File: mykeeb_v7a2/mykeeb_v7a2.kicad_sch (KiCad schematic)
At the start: 52 parts, among them SW43 SW_Push, SW44 SW_SPDT, U2 xiao-ble

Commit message: update
Signed-off-by: Maximilian Huber <gh@maxhbr.de>
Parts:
- added BT1: Battery_Cell, Connector_JST:JST_PH_S2B-PH-K_1x02_P2.00mm_Horizontal, symbol Device:Battery_Cell
- added D1, D11, D12, D13, D14, D15 (x2), D2, D3, D4 (x2), D6, D7, D8, D9: BAV70, Package_TO_SOT_SMD:SOT-23, symbol hillside_basic:BAV70_Small
- added S0, S1, S10, S11, S12, S13, S14, S15, S2, S20, S21, S22, S23, S24, S25, S3, S30 (x2), S31, S32, S33, S34, S35, S4, S43, S44, S45 (x2), S46: SW, pretty:MX-1U-Hotswap, symbol YAEMK:MX_1U
- added SW43: SW_Push, Button_Switch_SMD:SW_SPST_TL3342, symbol Switch:SW_Push
- added SW43: SW_Push, pretty:PushSW, symbol Switch:SW_Push
- added SW44: SW_SPDT, sepp:switch-MSK-12C02-smd, symbol Switch:SW_SPDT
- added U2: xiao-ble, pretty:xiao-ble-smd-cutout, symbol sepp:xiao-ble-geist
- SW43: footprint pretty:PushSW -> Button_Switch_SMD:SW_SPST_TL3342
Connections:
- net COL0: now also S0.2, S10.2, S20.2, S30.2, S30.2; no longer S0.1, S10.1, S20.1, S30.1, S30.1
- net COL1: now also S11.2, S21.1, S31.1, S43.1, SW43.1; no longer S11.1, S21.2, S31.2, S43.2, SW43.2
- net COL2: now also S12.1, S2.1, S22.2, S32.2, S44.2; no longer S12.2, S2.2, S22.1, S32.1, S44.1
- net COL3: now also S13.2, S23.1, S3.2, S33.1, S45.1; no longer S13.1, S23.2, S3.1, S33.2, S45.2
- net COL4: now also S14.1, S24.2, S34.2, S4.2, S46.2; no longer S14.2, S24.1, S34.1, S4.1, S46.1
- net COL5: now also S1.1, S15.2, S25.1, S35.1, S45.1; no longer S1.2, S15.1, S25.2, S35.2, S45.2
- net GND: now also BT1.2 (-), SW43.2, U2.13 (GND), U2.18 (GND), U2.20 (GND)
- net at D12.2 (A2): now also S15.1; no longer S15.2
- net at D4.1 (A1): now also S30.1; no longer S30.2 (x2)
- net at D4.2 (A2): now also S43.2; no longer S43.1
- net at D6.1 (A1): now also S2.2; no longer S2.1
- net at D6.2 (A2): now also S3.1; no longer S3.2
- net at D9.2 (A2): now also S33.2; no longer S33.1
- net at D2.2 (A2): now also S11.1; no longer S11.2
- net at D15.1 (A1): now also S44.1; no longer S44.2
- net at D12.1 (A1): now also S14.2; no longer S14.1
- net at D15.2 (A2): now also S45.2; no longer S45.1 (x2)
- net at D13.1 (A1): now also S24.1; no longer S24.2
- net at D13.2 (A2): now also S25.2; no longer S25.1
- net at D9.1 (A1): now also S32.1; no longer S32.2
- net at D2.1 (A1): now also S10.1; no longer S10.2
- net at D11.1 (A1): now also S4.1; no longer S4.2
- net at D11.2 (A2): now also S1.2; no longer S1.1
- net at D1.2 (A2): now also SW43.2; no longer SW43.1
- net at D8.1 (A1): now also S22.1; no longer S22.2
- net at D8.2 (A2): now also S23.2; no longer S23.1
- net at D14.1 (A1): now also S34.1; no longer S34.2
- net at D14.2 (A2): now also S35.2; no longer S35.1
- net at D3.1 (A1): now also S20.1; no longer S20.2
- net at D1.1 (A1): now also S0.1; no longer S0.2
- net at D15.1 (A1): now also S46.1; no longer S46.2
- net at D7.1 (A1): now also S12.2; no longer S12.1
- net at D4.2 (A2): now also S31.2; no longer S31.1
- net at D3.2 (A2): now also S21.2; no longer S21.1
- net at D7.2 (A2): now also S13.1; no longer S13.2
- new net: D8.1 (A1), S22.2
- new net: D8.2 (A2), S23.1
- new net: D12.2 (A2), S15.2
- new net: D11.1 (A1), S4.2
- new net: D4.1 (A1), S30.2 (x2)
- new net: D4.2 (A2), S43.1
- new net: D3.2 (A2), S21.1
- new net: D7.1 (A1), S12.1
- new net: D6.1 (A1), S2.1
- new net: D6.2 (A2), S3.2
- new net: D11.2 (A2), S1.1
- new net: D13.1 (A1), S24.2
- new net: D13.2 (A2), S25.1
- new net: D12.1 (A1), S14.1
- new net: D1.1 (A1), S0.2
- new net: D1.2 (A2), SW43.1
- new net: D14.2 (A2), S35.1
- new net: D2.1 (A1), S10.2
- new net: D2.2 (A2), S11.2
- new net: D7.2 (A2), S13.2
- new net: D15.2 (A2), S45.1 (x2)
- new net: D9.1 (A1), S32.2
- new net: D4.2 (A2), S31.1
- new net: D15.1 (A1), S46.2
- new net: D9.2 (A2), S33.1
- new net: D14.1 (A1), S34.2
- new net: D15.1 (A1), S44.2
- new net: D3.1 (A1), S20.2
- new net L_BAT+: SW44.2 (B), U2.19 (BAT)
- new net L_COL0: S0.1, S10.1, S20.1, S30.1, S30.1, U2.11 (A6_MOSI/1.15)
- new net L_COL1: S11.1, S21.2, S31.2, S43.2, SW43.2, U2.10 (A5_MISO/1.14)
- new net L_COL2: S12.2, S2.2, S22.1, S32.1, S44.1, U2.9 (A7_SCK/1.13)
- new net L_COL3: S13.1, S23.2, S3.1, S33.2, S45.2, U2.8 (B9_RX/1.12)
- new net L_COL4: S14.2, S24.1, S34.1, S4.1, S46.1, U2.7 (B8_TX/1.11)
- new net L_COL5: S1.2, S15.1, S25.2, S35.2, S45.2, U2.6 (A9_SCL/0.05_H)
- new net L_RESET: SW43.1, U2.17 (RESET)
- new net L_ROW0: D1.3 (K), D11.3 (K), D6.3 (K)
- new net L_ROW1: D12.3 (K), D2.3 (K), D7.3 (K), U2.1 (A2/0.02_H)
- new net L_ROW2: D13.3 (K), D3.3 (K), D8.3 (K), U2.2 (A4/0.03_H)
- new net L_ROW3: D14.3 (K), D4.3 (K), D9.3 (K), U2.3 (A10/0.28)
- new net L_ROW4: D15.3 (K), D15.3 (K), D4.3 (K), U2.4 (A11/0.29)
- new net L_ROW5: U2.5 (A8_SDA/0.04_H)
- new net L_VBAT: BT1.1 (+), SW44.3 (C)
- new net L_VCC: U2.12 (3V3)
- no-connect marks 4 -> 8
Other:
- moved on the sheet: BT1, D1, D11, D12, D13, D14, D15, D2, D3, D4, D6, D7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

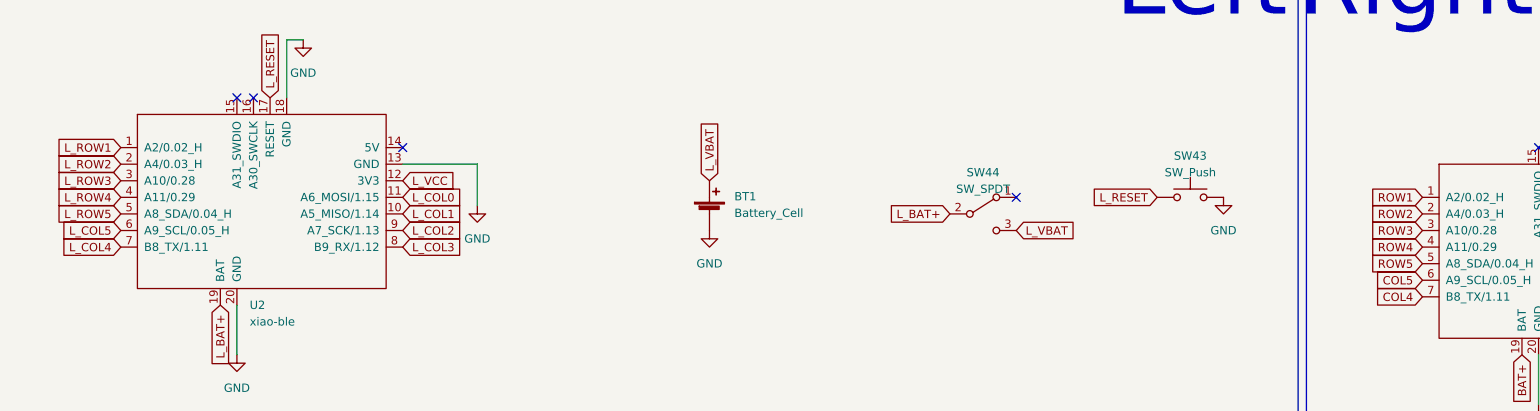
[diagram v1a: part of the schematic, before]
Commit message: routing
Signed-off-by: Maximilian Huber <gh@maxhbr.de>
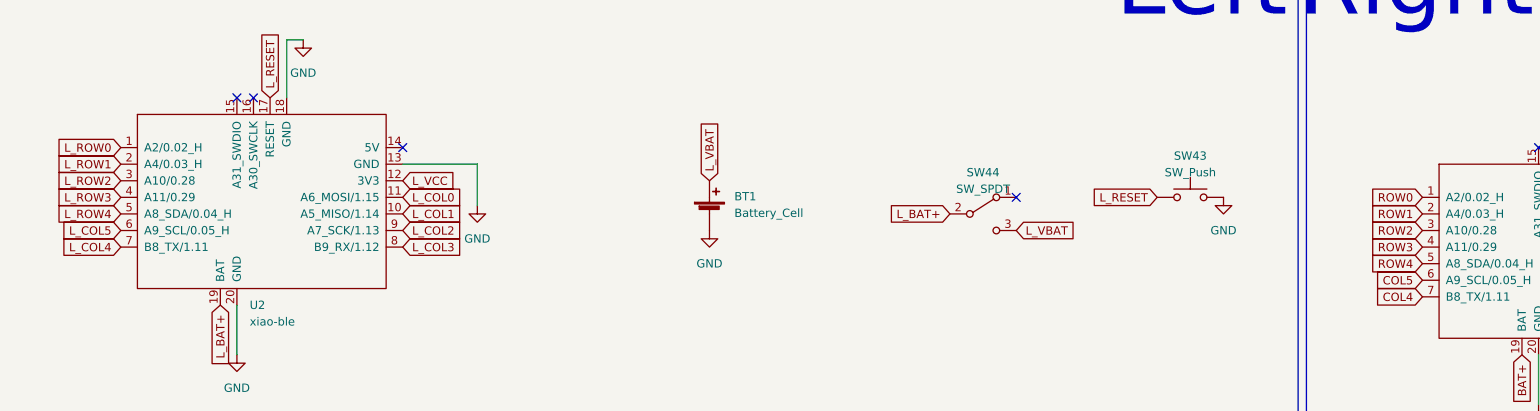
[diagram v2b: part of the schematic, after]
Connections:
- net L_ROW5 is gone; now on net L_ROW4: U2.5 (A8_SDA/0.04_H)
- net ROW5 is gone; now on net ROW4: U2.5 (A8_SDA/0.04_H)
- net L_ROW0: now also U2.1 (A2/0.02_H)
- net L_ROW1: now also U2.2 (A4/0.03_H); no longer U2.1 (A2/0.02_H)
- net L_ROW2: now also U2.3 (A10/0.28); no longer U2.2 (A4/0.03_H)
- net L_ROW3: now also U2.4 (A11/0.29); no longer U2.3 (A10/0.28)
- net L_ROW4: no longer U2.4 (A11/0.29)
- net ROW0: now also U2.1 (A2/0.02_H)
- net ROW1: now also U2.2 (A4/0.03_H); no longer U2.1 (A2/0.02_H)
- net ROW2: now also U2.3 (A10/0.28); no longer U2.2 (A4/0.03_H)
- net ROW3: now also U2.4 (A11/0.29); no longer U2.3 (A10/0.28)
- net ROW4: no longer U2.4 (A11/0.29)
